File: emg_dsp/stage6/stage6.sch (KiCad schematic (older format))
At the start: 169 parts, among them U1 RS232_CON, U10 EN_VDD, U11 USBLC6, U12 ABM10XTAL-24, U13 BF527, U14 AT25DF041-MHF, U15 ADSP_JTAG_CON, U16 LAN8710A, U17 74LCX541, U18 SFE-MAGJACK, U19 NRF24L01-BREAK, U2 VEE, U20 MAX6711Z, U21 TESTCON, U22 74LCX541, U23 74LCX541, U3 ADM3202, U4 TPS62410, U5 GT12MABE, U6 FCI_USB_B, U7 MT48LC16M16A2, U8 EN_VCC, U9 ABM10XTAL-25

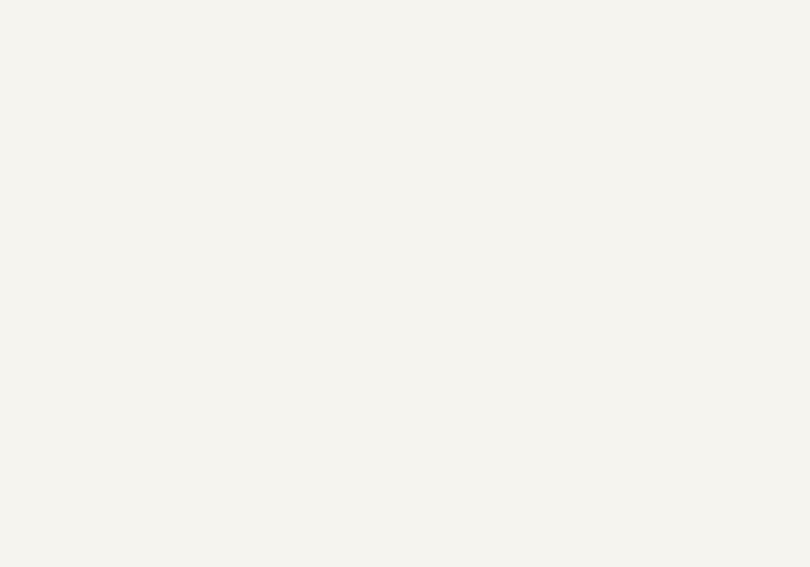
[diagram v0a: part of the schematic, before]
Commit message: board getting done! next up is silkscreen - pita.
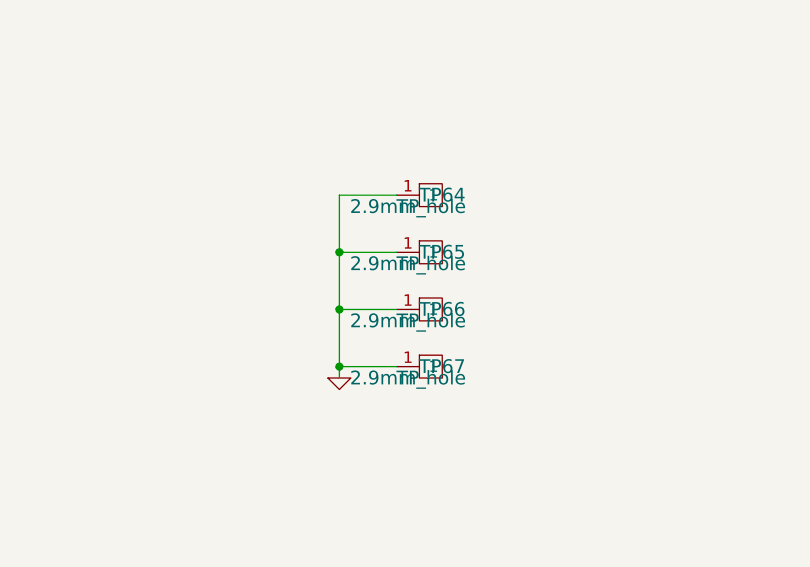
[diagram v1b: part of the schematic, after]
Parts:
- added TP64, TP65, TP66, TP67: TP, 2.9mm_hole, symbol TP
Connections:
- net GND: now also TP64.1, TP65.1, TP66.1, TP67.1
